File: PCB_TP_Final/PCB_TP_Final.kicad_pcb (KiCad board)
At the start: 2 copper layers, 6 parts, among them CN10 Conn_02x17_Odd_Even, CN7 Conn_02x10_Odd_Even, CN8 Conn_02x08_Odd_Even, CN9 Conn_02x15_Odd_Even, J1 Conn_01x09, U1 NODEMCU_ESP12

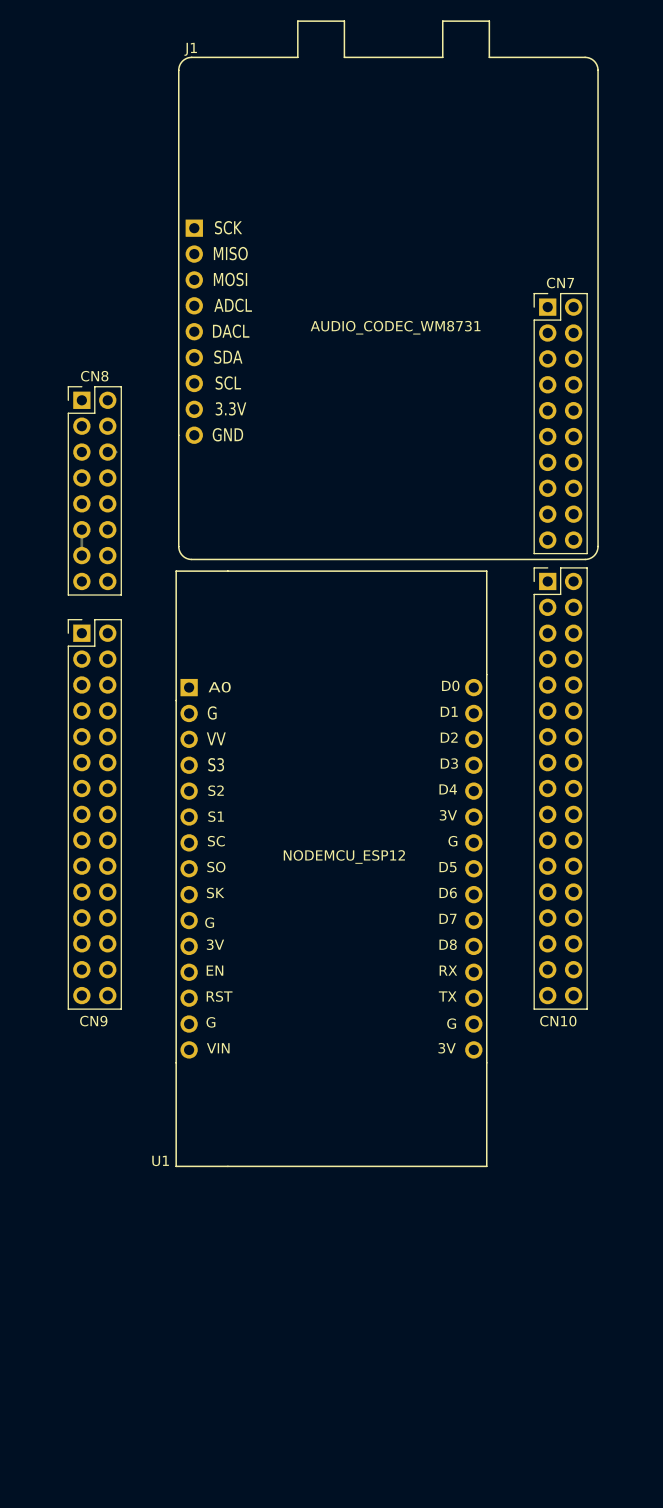
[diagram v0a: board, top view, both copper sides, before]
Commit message: Primera entrega (1.0) para revision
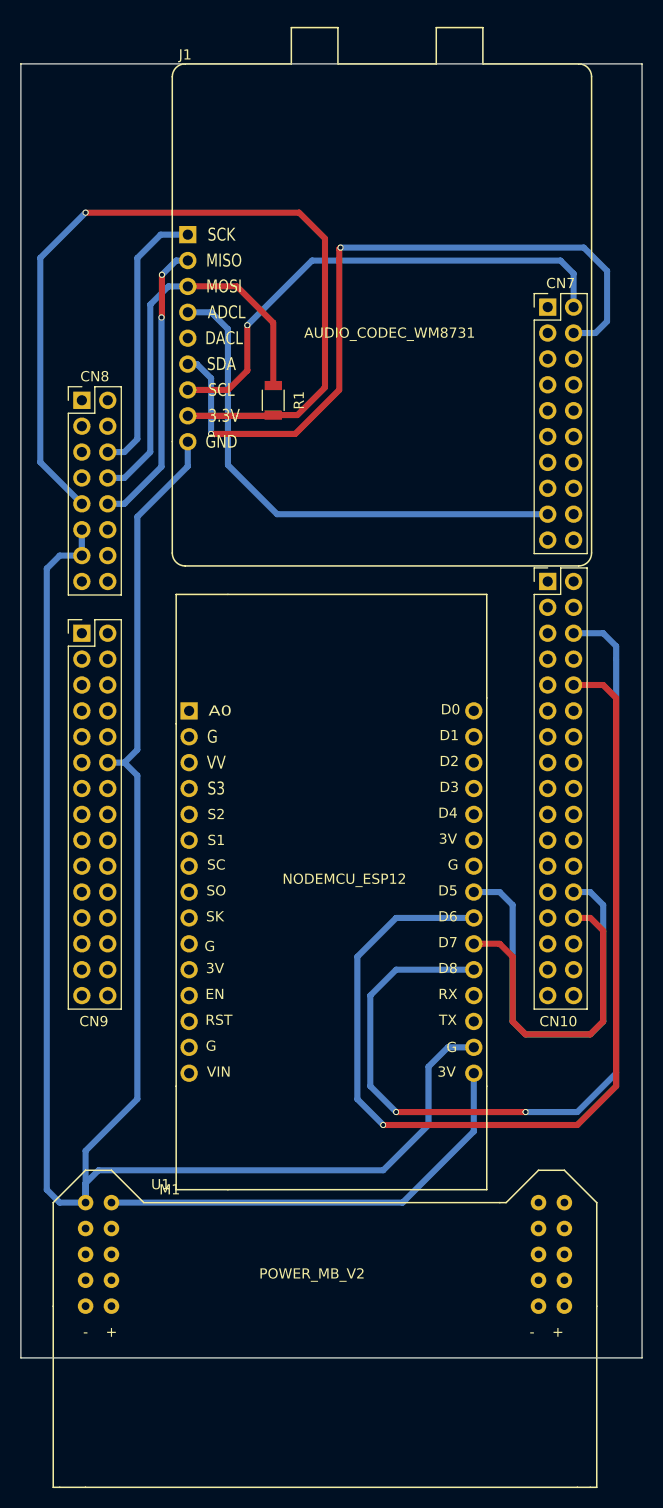
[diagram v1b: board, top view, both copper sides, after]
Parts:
- added M1: POWER_MB_V2, POWER_MB_V2:POWER_MB_V2, F.Cu at (124.5, 167.6)
- added R1: 3.3K, Resistors_SMD:R_1206, F.Cu at (120.0, 83.8)
- moved U1 2.29 mm to (127.0, 132.1)
- moved J1 0.90 mm to (131.4, 78.7)
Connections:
- CN10 pad 10: Net-(CN10-Pad10) -> /NODEMCU_ESP12/HMISO
- CN10 pad 26: Net-(CN10-Pad26) -> /NODEMCU_ESP12/HSCLK
- CN10 pad 28: Net-(CN10-Pad28) -> /NODEMCU_ESP12/HMOSI
- CN10 pad 6: Net-(CN10-Pad6) -> /NODEMCU_ESP12/HCS
- CN8 pad 9: +3V3 -> 3.3VB
- CN9 pad 12: Net-(CN9-Pad12) -> GND
- J1 pad 8: +3V3 -> 3.3VB
- U1 pad 16: Net-(U1-Pad16) -> +3V3
- U1 pad 20: Net-(U1-Pad20) -> /NODEMCU_ESP12/HCS
- U1 pad 21: Net-(U1-Pad21) -> /NODEMCU_ESP12/HMOSI
- U1 pad 22: Net-(U1-Pad22) -> /NODEMCU_ESP12/HMISO
- U1 pad 23: Net-(U1-Pad23) -> /NODEMCU_ESP12/HSCLK
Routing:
- net GND: track 2.54 -> 202.2 mm
- net /NODEMCU_ESP12/HMISO: track 0.00 -> 97.8 mm, vias 0 -> 1
- net /NODEMCU_ESP12/HCS: track 0.00 -> 93.5 mm, vias 0 -> 2
- net 3.3VB: track 0.00 -> 85.9 mm, vias 0 -> 1
- net /AUDIO_CODEC/SDA: track 0.00 -> 72.5 mm, vias 0 -> 2
- net /AUDIO_CODEC/ADCL: track 0.00 -> 51.3 mm
- net /AUDIO_CODEC/SCL: track 0.00 -> 49.5 mm, vias 0 -> 1
- net +3V3: track 0.00 -> 44.2 mm
- net /NODEMCU_ESP12/HSCLK: track 0.00 -> 40.6 mm
- net /AUDIO_CODEC/MOSI: track 0.00 -> 40.2 mm
- net /NODEMCU_ESP12/HMOSI: track 0.00 -> 32.9 mm
- net /AUDIO_CODEC/MISO: track 0.00 -> 28.8 mm, vias 0 -> 2
- net /AUDIO_CODEC/SCK: track 0.84 -> 27.9 mm
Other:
- board outline added: 61 x 127 mm
- net class Default: clearance 0.2 -> 0.4; trace_width 0.25 -> 0.6
- rule trace_clearance: 0.2 -> 0.4
